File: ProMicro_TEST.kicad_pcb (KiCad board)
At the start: 2 copper layers, 17.8 x 30.5 mm, 6 parts

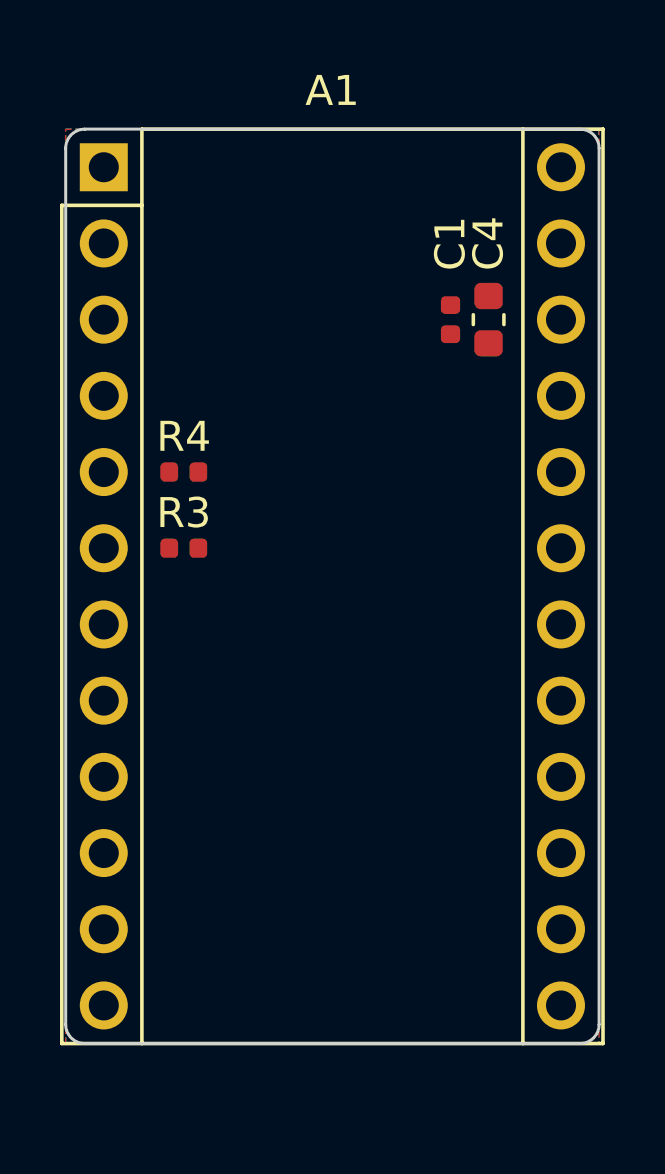
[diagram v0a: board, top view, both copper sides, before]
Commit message: test
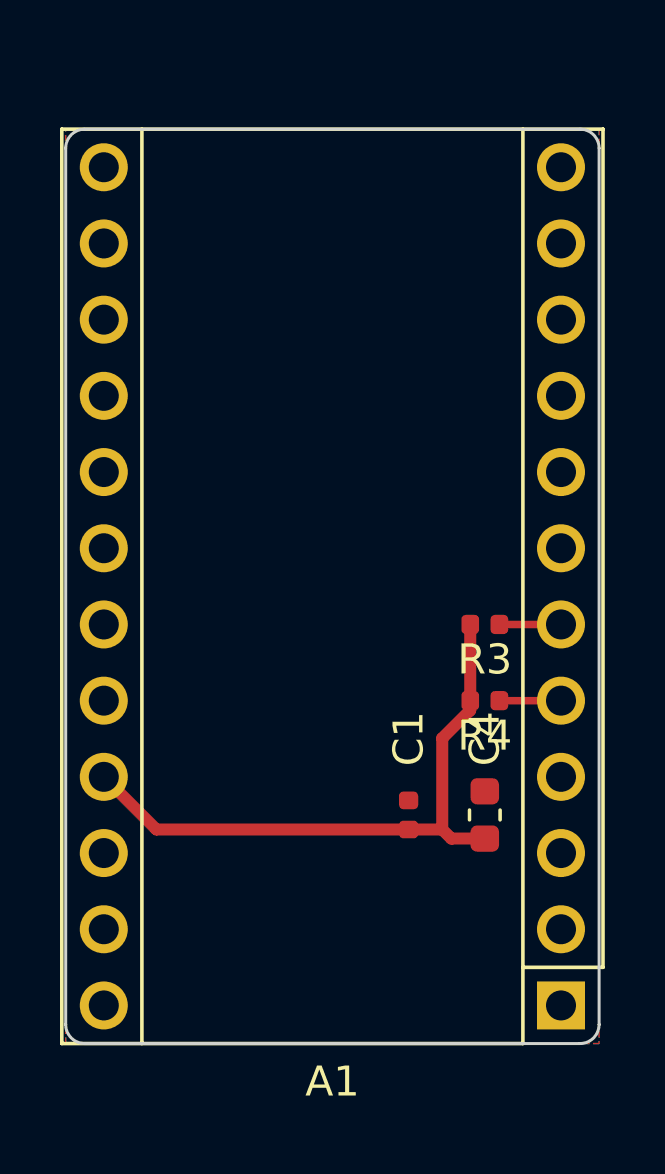
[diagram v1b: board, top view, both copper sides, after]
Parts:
- moved A1 31.8 mm to (152.4, 114.3), turned to 180 degrees
- moved C1 16.6 mm to (147.3, 108.0)
- moved C4 16.5 mm to (149.9, 108.0)
- moved R4 12.6 mm to (149.9, 104.1), turned to 180 degrees
- moved R3 10.3 mm to (149.9, 101.6), turned to 180 degrees
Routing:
- net +3V3: track 0.00 -> 20.8 mm
- net SDA: track 0.00 -> 2.06 mm
- net SCL: track 0.00 -> 2.06 mm
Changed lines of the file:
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@@
     (thickness 0.8)
     (drawings 62)
-    (tracks 0)
+    (tracks 11)
     (zones 0)
     (modules 6)
@@
   )
   (setup
-    (last_trace_width 0.25)
+    (last_trace_width 0.1)
     (user_trace_width 0.1)
     (user_trace_width 0.2)
@@
     (uvia_dia 0.3)
     (uvia_drill 0.1)
-    (add_net A0)
-    (add_net A1)
-    (add_net A2)
-    (add_net A3)
-    (add_net D10)
-    (add_net D4)
-    (add_net D5)
-    (add_net D6)
-    (add_net D7)
-    (add_net D8)
-    (add_net D9)
-    (add_net MISO)
-    (add_net MOSI)
-    (add_net "Net-(A1-Pad24)")
-    (add_net "Net-(A1-Pad3)")
-    (add_net RXD)
-    (add_net Reset)
-    (add_net SCK)
     (add_net SCL)
     (add_net SDA)
-    (add_net TXD)
   )
   (net_class Power ""
@@
   )
   (module Module:Sparkfun_Pro_Micro (layer F.Cu)
-    (at 137.16 86.36)
+    (at 152.4 114.3 180)
     (descr "Sparkfun Pro Micro, https://www.sparkfun.com/products/12587")
     (tags "Sparkfun Pro Micro")
@@
     (fp_line (start 16.8 29.3) (end 16.8 -1.5) (layer F.CrtYd) (width 0.05))
     (fp_line (start 16.8 29.3) (end -1.5 29.3) (layer F.CrtYd) (width 0.05))
-    (pad 24 thru_hole oval (at 15.24 0) (size 1.6 1.6) (drill 1) (layers *.Cu *.Mask))
-    (pad 23 thru_hole oval (at 15.24 2.54) (size 1.6 1.6) (drill 1) (layers *.Cu *.Mask)
+    (pad 24 thru_hole oval (at 15.24 0 180) (size 1.6 1.6) (drill 1) (layers *.Cu *.Mask))
+    (pad 23 thru_hole oval (at 15.24 2.54 180) (size 1.6 1.6) (drill 1) (layers *.Cu *.Mask)
       (net 1 GND))
-    (pad 22 thru_hole oval (at 15.24 5.08) (size 1.6 1.6) (drill 1) (layers *.Cu *.Mask))
-    (pad 12 thru_hole oval (at 0 27.94) (size 1.6 1.6) (drill 1) (layers *.Cu *.Mask))
-    (pad 21 thru_hole oval (at 15.24 7.62) (size 1.6 1.6) (drill 1) (layers *.Cu *.Mask)
+    (pad 22 thru_hole oval (at 15.24 5.08 180) (size 1.6 1.6) (drill 1) (layers *.Cu *.Mask))
+    (pad 12 thru_hole oval (at 0 27.94 180) (size 1.6 1.6) (drill 1) (layers *.Cu *.Mask))
+    (pad 21 thru_hole oval (at 15.24 7.62 180) (size 1.6 1.6) (drill 1) (layers *.Cu *.Mask)
       (net 2 +3V3))
-    (pad 11 thru_hole oval (at 0 25.4) (size 1.6 1.6) (drill 1) (layers *.Cu *.Mask))
-    (pad 20 thru_hole oval (at 15.24 10.16) (size 1.6 1.6) (drill 1) (layers *.Cu *.Mask))
-    (pad 10 thru_hole oval (at 0 22.86) (size 1.6 1.6) (drill 1) (layers *.Cu *.Mask))
-    (pad 19 thru_hole oval (at 15.24 12.7) (size 1.6 1.6) (drill 1) (layers *.Cu *.Mask))
-    (pad 9 thru_hole oval (at 0 20.32) (size 1.6 1.6) (drill 1) (layers *.Cu *.Mask))
-    (pad 18 thru_hole oval (at 15.24 15.24) (size 1.6 1.6) (drill 1) (layers *.Cu *.Mask))
-    (pad 8 thru_hole oval (at 0 17.78) (size 1.6 1.6) (drill 1) (layers *.Cu *.Mask))
-    (pad 17 thru_hole oval (at 15.24 17.78) (size 1.6 1.6) (drill 1) (layers *.Cu *.Mask))
-    (pad 7 thru_hole oval (at 0 15.24) (size 1.6 1.6) (drill 1) (layers *.Cu *.Mask))
-    (pad 16 thru_hole oval (at 15.24 20.32) (size 1.6 1.6) (drill 1) (layers *.Cu *.Mask))
-    (pad 6 thru_hole oval (at 0 12.7) (size 1.6 1.6) (drill 1) (layers *.Cu *.Mask)
+    (pad 11 thru_hole oval (at 0 25.4 180) (size 1.6 1.6) (drill 1) (layers *.Cu *.Mask))
+    (pad 20 thru_hole oval (at 15.24 10.16 180) (size 1.6 1.6) (drill 1) (layers *.Cu *.Mask))
+    (pad 10 thru_hole oval (at 0 22.86 180) (size 1.6 1.6) (drill 1) (layers *.Cu *.Mask))
+    (pad 19 thru_hole oval (at 15.24 12.7 180) (size 1.6 1.6) (drill 1) (layers *.Cu *.Mask))
+    (pad 9 thru_hole oval (at 0 20.32 180) (size 1.6 1.6) (drill 1) (layers *.Cu *.Mask))
+    (pad 18 thru_hole oval (at 15.24 15.24 180) (size 1.6 1.6) (drill 1) (layers *.Cu *.Mask))
+    (pad 8 thru_hole oval (at 0 17.78 180) (size 1.6 1.6) (drill 1) (layers *.Cu *.Mask))
+    (pad 17 thru_hole oval (at 15.24 17.78 180) (size 1.6 1.6) (drill 1) (layers *.Cu *.Mask))
+    (pad 7 thru_hole oval (at 0 15.24 180) (size 1.6 1.6) (drill 1) (layers *.Cu *.Mask))
+    (pad 16 thru_hole oval (at 15.24 20.32 180) (size 1.6 1.6) (drill 1) (layers *.Cu *.Mask))
+    (pad 6 thru_hole oval (at 0 12.7 180) (size 1.6 1.6) (drill 1) (layers *.Cu *.Mask)
       (net 3 SCL))
-    (pad 15 thru_hole oval (at 15.24 22.86) (size 1.6 1.6) (drill 1) (layers *.Cu *.Mask))
-    (pad 5 thru_hole oval (at 0 10.16) (size 1.6 1.6) (drill 1) (layers *.Cu *.Mask)
+    (pad 15 thru_hole oval (at 15.24 22.86 180) (size 1.6 1.6) (drill 1) (layers *.Cu *.Mask))
+    (pad 5 thru_hole oval (at 0 10.16 180) (size 1.6 1.6) (drill 1) (layers *.Cu *.Mask)
       (net 4 SDA))
-    (pad 14 thru_hole oval (at 15.24 25.4) (size 1.6 1.6) (drill 1) (layers *.Cu *.Mask))
-    (pad 4 thru_hole oval (at 0 7.62) (size 1.6 1.6) (drill 1) (layers *.Cu *.Mask)
+    (pad 14 thru_hole oval (at 15.24 25.4 180) (size 1.6 1.6) (drill 1) (layers *.Cu *.Mask))
+    (pad 4 thru_hole oval (at 0 7.62 180) (size 1.6 1.6) (drill 1) (layers *.Cu *.Mask)
       (net 1 GND))
-    (pad 13 thru_hole oval (at 15.24 27.94) (size 1.6 1.6) (drill 1) (layers *.Cu *.Mask))
-    (pad 3 thru_hole oval (at 0 5.08) (size 1.6 1.6) (drill 1) (layers *.Cu *.Mask))
-    (pad 2 thru_hole oval (at 0 2.54) (size 1.6 1.6) (drill 1) (layers *.Cu *.Mask))
-    (pad 1 thru_hole rect (at 0 0) (size 1.6 1.6) (drill 1) (layers *.Cu *.Mask))
+    (pad 13 thru_hole oval (at 15.24 27.94 180) (size 1.6 1.6) (drill 1) (layers *.Cu *.Mask))
+    (pad 3 thru_hole oval (at 0 5.08 180) (size 1.6 1.6) (drill 1) (layers *.Cu *.Mask))
+    (pad 2 thru_hole oval (at 0 2.54 180) (size 1.6 1.6) (drill 1) (layers *.Cu *.Mask))
+    (pad 1 thru_hole rect (at 0 0 180) (size 1.6 1.6) (drill 1) (layers *.Cu *.Mask))
     (model ${KISYS3DMOD}/Module.3dshapes/Sparkfun_Pro_Micro.wrl
       (at (xyz 0 0 0))
@@
   )
   (module Resistor_SMD:R_0402_1005Metric (layer F.Cu)
-    (at 139.827 96.52)
+    (at 149.86 104.14 180)
     (descr "Resistor SMD 0402 (1005 Metric), square (rectangular) end terminal, IPC_7351 nominal, (Body size source: http://www.tortai-tech.com/upload/download/2011102023233369053.pdf), generated with kicad-footprint-generator")
     (tags resistor)
@@
     (fp_line (start -0.5 -0.25) (end 0.5 -0.25) (layer F.Fab) (width 0.1))
     (fp_line (start -0.5 0.25) (end -0.5 -0.25) (layer F.Fab) (width 0.1))
-    (pad 2 smd roundrect (at 0.485 0) (size 0.59 0.64) (layers F.Cu F.Paste F.Mask) (roundrect_rratio 0.25)
+    (pad 2 smd roundrect (at 0.485 0 180) (size 0.59 0.64) (layers F.Cu F.Paste F.Mask) (roundrect_rratio 0.25)
       (net 2 +3V3))
-    (pad 1 smd roundrect (at -0.485 0) (size 0.59 0.64) (layers F.Cu F.Paste F.Mask) (roundrect_rratio 0.25)
+    (pad 1 smd roundrect (at -0.485 0 180) (size 0.59 0.64) (layers F.Cu F.Paste F.Mask) (roundrect_rratio 0.25)
       (net 4 SDA))
     (model ${KISYS3DMOD}/Resistor_SMD.3dshapes/R_0402_1005Metric.wrl
@@
   )
   (module Resistor_SMD:R_0402_1005Metric (layer F.Cu)
-    (at 139.827 99.06)
+    (at 149.86 101.6 180)
     (descr "Resistor SMD 0402 (1005 Metric), square (rectangular) end terminal, IPC_7351 nominal, (Body size source: http://www.tortai-tech.com/upload/download/2011102023233369053.pdf), generated with kicad-footprint-generator")
     (tags resistor)
@@
     (fp_line (start -0.5 -0.25) (end 0.5 -0.25) (layer F.Fab) (width 0.1))
     (fp_line (start -0.5 0.25) (end -0.5 -0.25) (layer F.Fab) (width 0.1))
-    (pad 2 smd roundrect (at 0.485 0) (size 0.59 0.64) (layers F.Cu F.Paste F.Mask) (roundrect_rratio 0.25)
+    (pad 2 smd roundrect (at 0.485 0 180) (size 0.59 0.64) (layers F.Cu F.Paste F.Mask) (roundrect_rratio 0.25)
       (net 2 +3V3))
-    (pad 1 smd roundrect (at -0.485 0) (size 0.59 0.64) (layers F.Cu F.Paste F.Mask) (roundrect_rratio 0.25)
+    (pad 1 smd roundrect (at -0.485 0 180) (size 0.59 0.64) (layers F.Cu F.Paste F.Mask) (roundrect_rratio 0.25)
       (net 3 SCL))
     (model ${KISYS3DMOD}/Resistor_SMD.3dshapes/R_0402_1005Metric.wrl
@@
   )
   (module Capacitor_SMD:C_0603_1608Metric (layer F.Cu)
-    (at 149.987 91.44 90)
+    (at 149.86 107.95 90)
     (descr "Capacitor SMD 0603 (1608 Metric), square (rectangular) end terminal, IPC_7351 nominal, (Body size source: http://www.tortai-tech.com/upload/download/2011102023233369053.pdf), generated with kicad-footprint-generator")
     (tags capacitor)
@@
   )
   (module Capacitor_SMD:C_0402_1005Metric (layer F.Cu)
-    (at 148.717 91.44 90)
+    (at 147.32 107.95 90)
     (descr "Capacitor SMD 0402 (1005 Metric), square (rectangular) end terminal, IPC_7351 nominal, (Body size source: http://www.tortai-tech.com/upload/download/2011102023233369053.pdf), generated with kicad-footprint-generator")
     (tags capacitor)
@@
   (gr_line (start 153.035 115.57) (end 136.525 115.57) (layer Edge.Cuts) (width 0.1))
   (gr_line (start 136.525 85.09) (end 153.035 85.09) (layer Edge.Cuts) (width 0.1))
+  (segment (start 149.375 101.6) (end 149.375 104.14) (width 0.4) (layer F.Cu) (net 2))
+  (segment (start 149.86 108.7375) (end 148.7425 108.7375) (width 0.4) (layer F.Cu) (net 2))
+  (segment (start 148.44 108.435) (end 147.32 108.435) (width 0.4) (layer F.Cu) (net 2))
+  (segment (start 148.7425 108.7375) (end 148.44 108.435) (width 0.4) (layer F.Cu) (net 2))
+  (segment (start 138.915 108.435) (end 137.16 106.68) (width 0.4) (layer F.Cu) (net 2))
+  (segment (start 147.32 108.435) (end 138.915 108.435) (width 0.4) (layer F.Cu) (net 2))
+  (segment (start 148.44 105.395) (end 148.44 108.435) (width 0.4) (layer F.Cu) (net 2) (status 1000000))
+  (segment (start 149.375 104.14) (end 149.375 104.46) (width 0.4) (layer F.Cu) (net 2) (status 1000000))
+  (segment (start 149.375 104.46) (end 148.44 105.395) (width 0.4) (layer F.Cu) (net 2) (status 1000000))
+  (segment (start 152.4 101.6) (end 150.345 101.6) (width 0.25) (layer F.Cu) (net 3))
+  (segment (start 150.345 104.14) (end 152.4 104.14) (width 0.25) (layer F.Cu) (net 4))
   (zone (net 1) (net_name GND) (layer F.Cu) (hatch edge 0.508)
     (connect_pads (clearance 0.125))

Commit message: drc
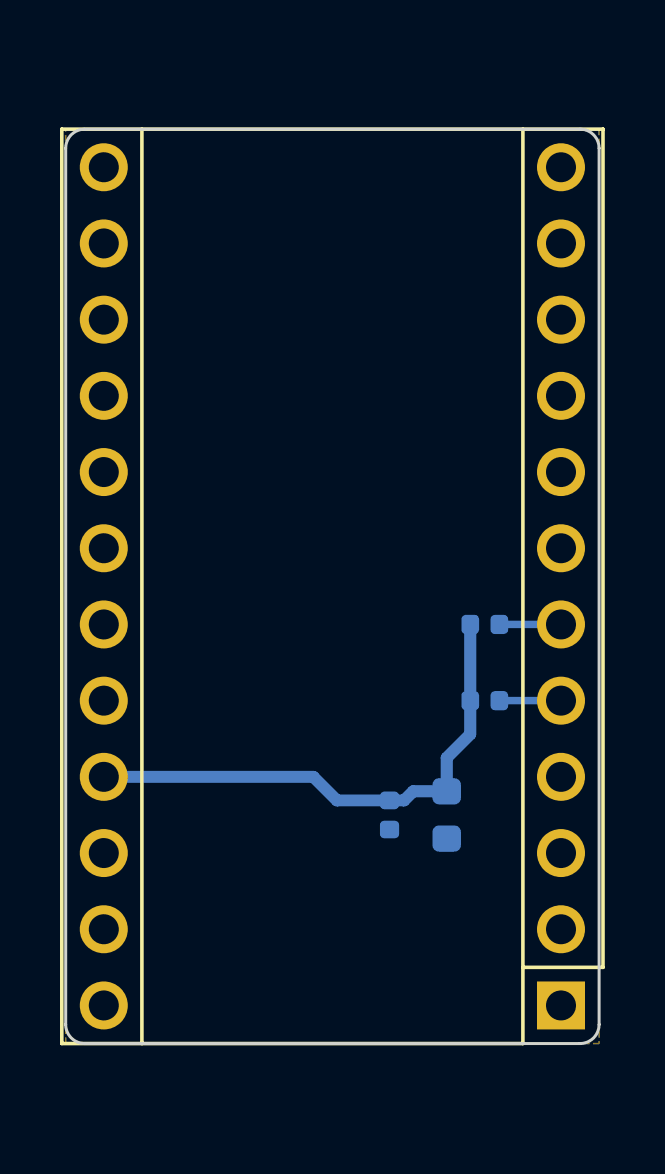
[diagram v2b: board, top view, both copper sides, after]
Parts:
- C1, C4, R3, R4: moved to B.Cu
- moved C4 1.27 mm to (148.6, 108.0), turned to 270 degrees
- moved LOGO1 1.27 mm to (144.1, 100.3)
- moved C1 0.63 mm to (146.7, 108.0), turned to 270 degrees
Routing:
- net +3V3: track 20.8 -> 17.8 mm
